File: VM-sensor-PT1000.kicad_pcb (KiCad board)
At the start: 2 copper layers, 26 x 24.8 mm, 20 parts, among them P1 PT100, P2 ADC, P3 PWR, U1 AMS1117, U2 MCP6001

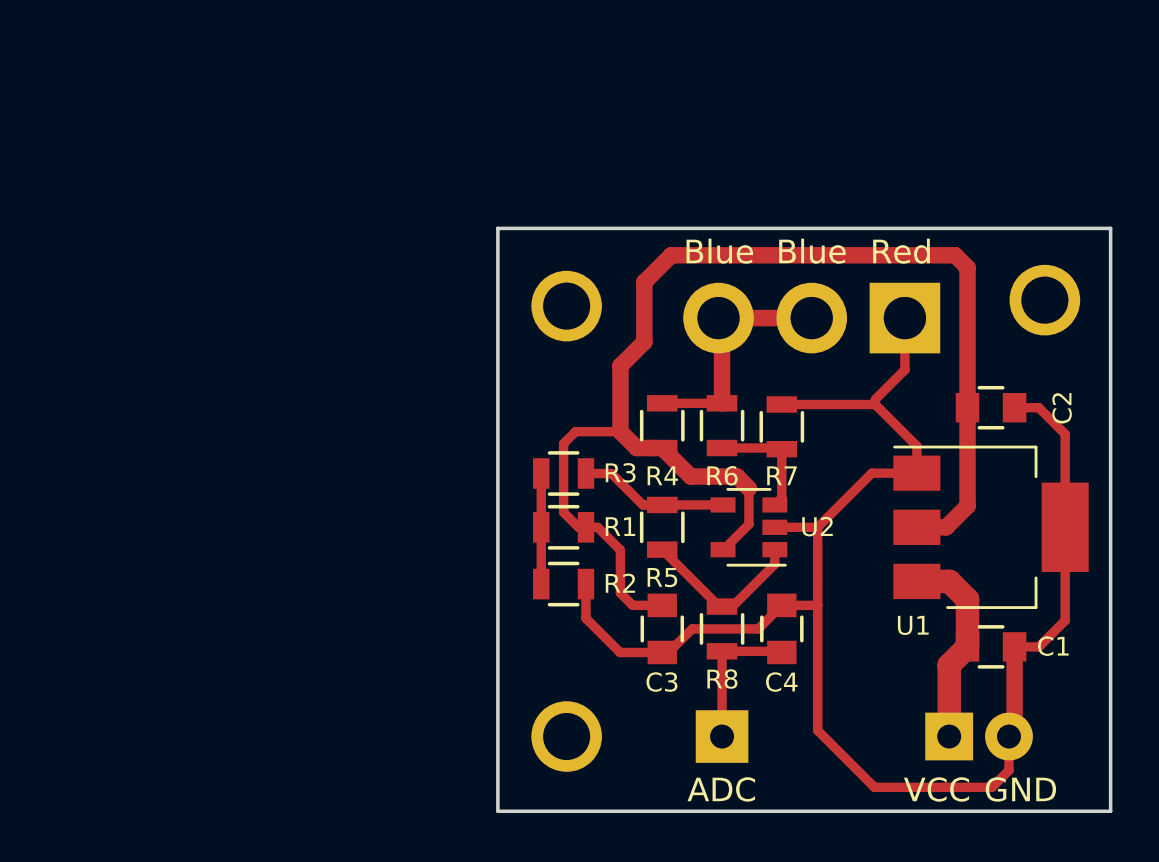
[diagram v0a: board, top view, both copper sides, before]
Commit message: completed new PCB design
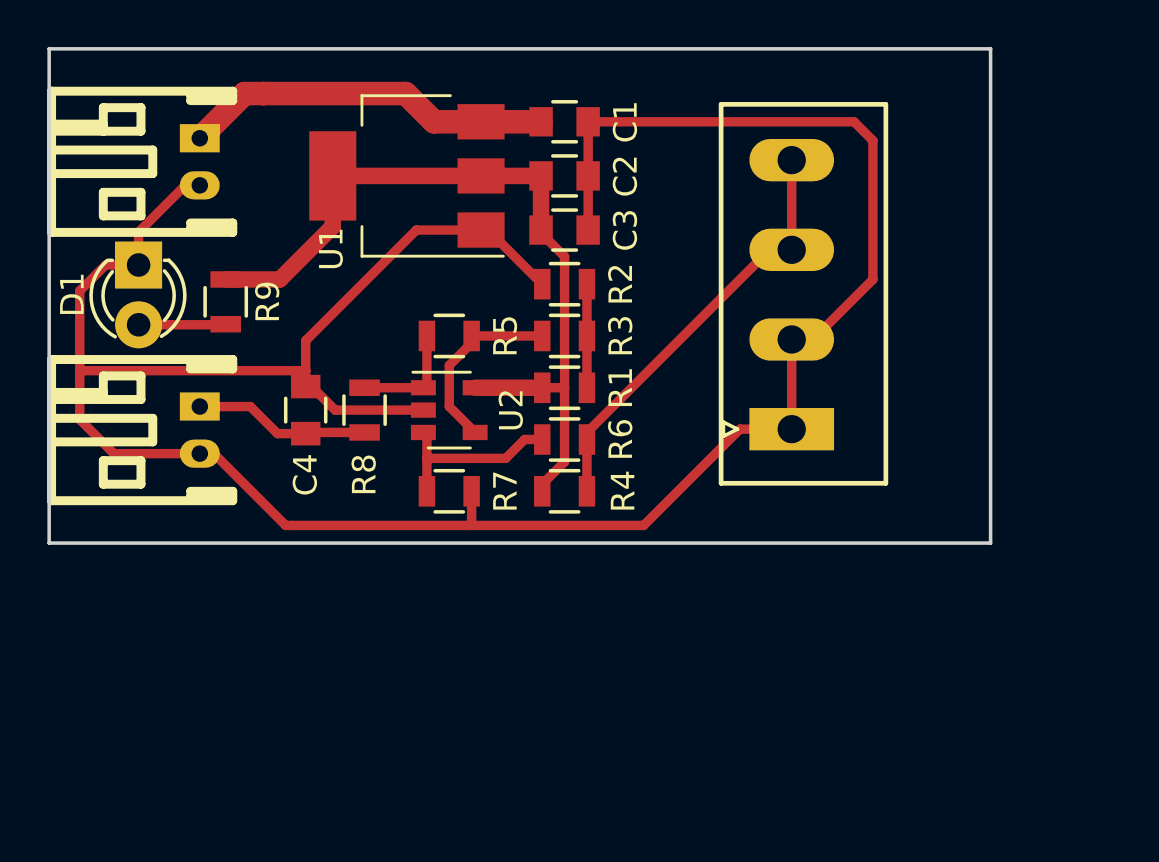
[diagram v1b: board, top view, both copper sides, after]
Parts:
- removed P1: PT100, Connectors_Hirose:Hirose_DF63-3P-3.96DSA_03x3.96mm_Straight
- removed REF** (x3): SolderWirePad_single_1-2mmDrill, Wire_Pads:SolderWirePad_single_1-2mmDrill
- added D1: LED_Small, LEDs:LED-3MM, F.Cu at (123.8, 89.2)
- added PT100: PT100, lib:Domino-PT100.pretty, F.Cu at (151.6, 96.2)
- added R9: 100R/1%, Resistors_SMD:R_0805, F.Cu at (127.5, 90.8)
- C3: value lib:C_0603 -> 10uF
- P2: footprint Pin_Headers:Pin_Header_Straight_1x01 -> w_conn_jst-ph:s2b-ph-kl
- P3: footprint Pin_Headers:Pin_Header_Straight_1x02 -> w_conn_jst-ph:s2b-ph-kl
- R2: value 100/1% -> 100R/1%
- R3, R6: value 1K/1% -> 16.9K/1%
- R5, R7: value 100K/1% -> 1M/1%
- U2: value MCP6001 -> MCP601T
- moved P3 40.1 mm to (126.4, 84.8), turned to 270 degrees
- moved U1 29.0 mm to (135.2, 85.4), turned to 180 degrees
- moved C1 28.7 mm to (141.9, 83.1)
- moved P2 25.7 mm to (126.4, 96.2)
- moved C4 22.3 mm to (130.9, 95.3)
- moved C2 20.6 mm to (141.9, 85.4)
- moved R8 17.8 mm to (133.4, 95.3)
- moved C3 17.4 mm to (141.9, 87.7), turned to 0 degrees
- moved R7 14.4 mm to (137.0, 98.8), turned to 180 degrees
- moved U2 13.7 mm to (137.0, 95.3), turned to 0 degrees
- moved R2 12.7 mm to (141.9, 90.0), turned to 180 degrees
- moved R5 12.2 mm to (137.0, 92.2), turned to 180 degrees
- moved R6 6.72 mm to (141.9, 96.6), turned to 0 degrees
- moved R1 5.93 mm to (141.9, 94.4), turned to 0 degrees
- moved R3 5.84 mm to (141.9, 92.2), turned to 0 degrees
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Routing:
- net GND: track 68.1 -> 110.0 mm
- net +3V3: track 55.9 -> 34.5 mm
- net /Blue: track 10.2 -> 18.2 mm
- net VCC: track 8.61 -> 15.8 mm
- net Net-(D1-Pad2): track 0.00 -> 4.12 mm
- net Net-(R6-Pad1): track 5.05 -> 7.79 mm
- net Net-(R5-Pad2): track 7.27 -> 4.76 mm
- net Net-(R3-Pad1): track 6.38 -> 7.95 mm
- net /ADC: track 6.18 -> 7.50 mm
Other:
- board size 26 x 24.8 mm -> 40 x 21 mm
- net class Default: trace_width 0.7 -> 1
- board text added: "+"
- board text added: "-"
- board text added: "BLUE"
- board text added: "PWR"
- board text added: "RED"
- board text removed: "ADC"
- board text removed: "Blue"
- board text removed: "GND"
- board text removed: "Red"
- board text removed: "VCC"
